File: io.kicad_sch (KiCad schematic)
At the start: 48 parts

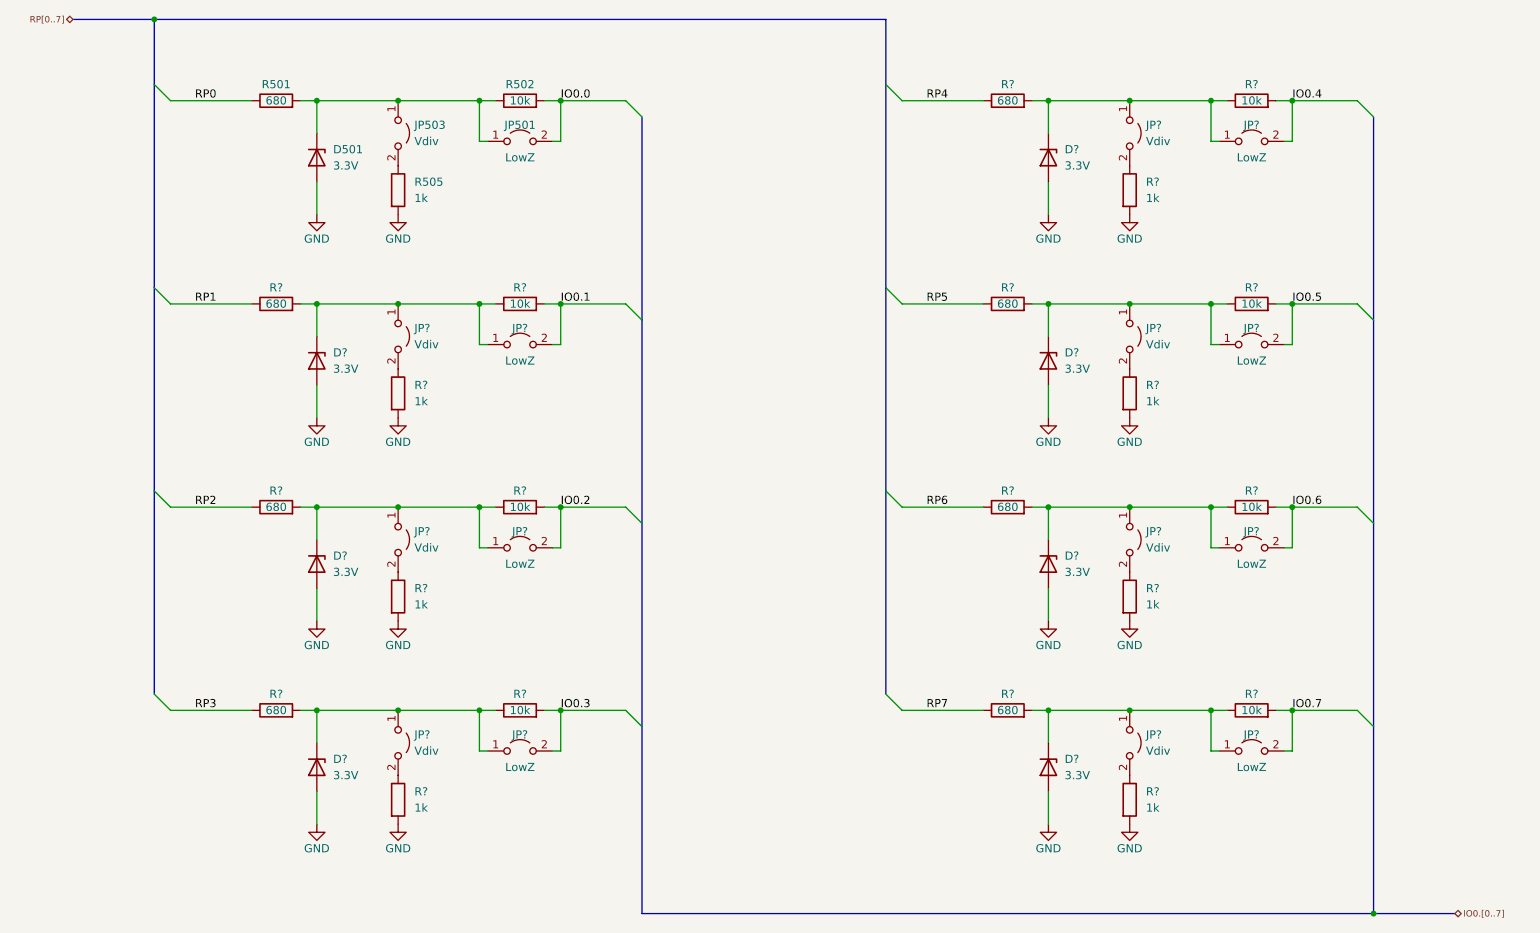
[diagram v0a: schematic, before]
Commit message: started routing
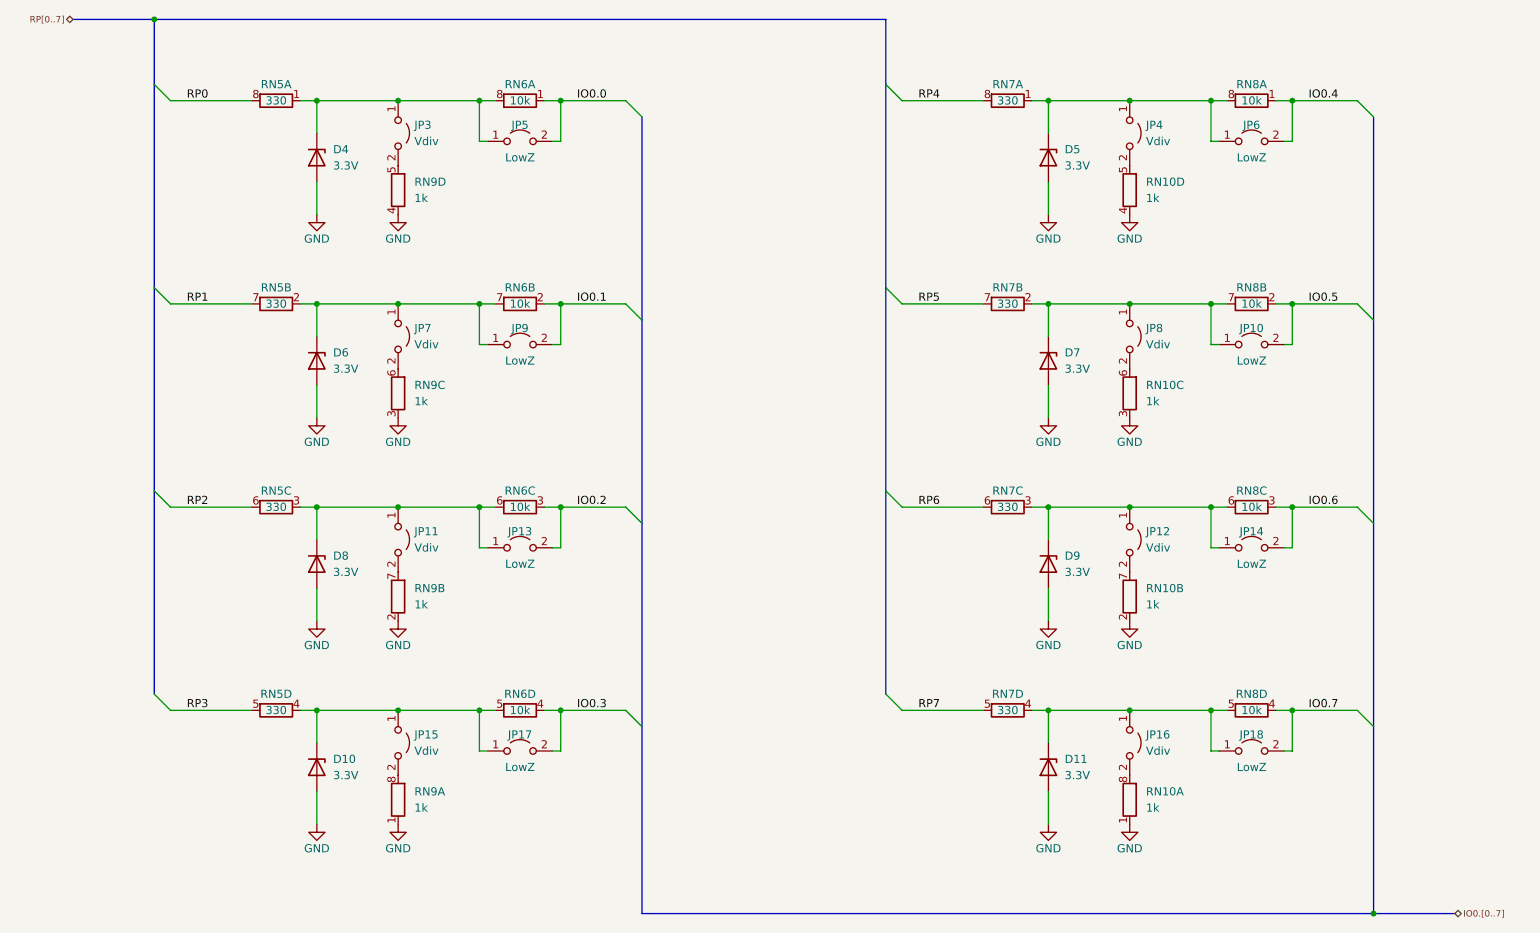
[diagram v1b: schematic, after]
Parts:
- removed D? (x4): 3.3V, symbol Device:D_Zener
- removed JP? (x4): LowZ, symbol Jumper:Jumper_2_Open
- removed JP? (x4): Vdiv, symbol Jumper:Jumper_2_Open
- removed R501, R? (x7): 680, symbol Device:R
- removed R502, R? (x7): 10k, symbol Device:R
- removed R505, R? (x7): 1k, symbol Device:R
- added D11, D5, D7, D9: 3.3V, Diode_SMD:D_SOD-123, symbol Device:D_Zener
- added JP10, JP14, JP18, JP6: LowZ, Jumper:SolderJumper-2_P1.3mm_Open_TrianglePad1.0x1.5mm, symbol Jumper:Jumper_2_Open
- added JP12, JP16, JP4, JP8: Vdiv, Jumper:SolderJumper-2_P1.3mm_Open_TrianglePad1.0x1.5mm, symbol Jumper:Jumper_2_Open
- added RN10, RN9: 1k, Resistor_SMD:R_Array_Convex_4x0603, symbol Device:R_Pack04_Split
- added RN5, RN7: 330, Resistor_SMD:R_Array_Convex_4x0603, symbol Device:R_Pack04_Split
- added RN6, RN8: 10k, Resistor_SMD:R_Array_Convex_4x0603, symbol Device:R_Pack04_Split
- D10, D6, D8: renamed from D?; footprint (none) -> Diode_SMD:D_SOD-123
- D4: renamed from D501; footprint (none) -> Diode_SMD:D_SOD-123
- JP11, JP13, JP15, JP17, JP7, JP9: renamed from JP?; footprint (none) -> Jumper:SolderJumper-2_P1.3mm_Open_TrianglePad1.0x1.5mm
- JP3: renamed from JP503; footprint (none) -> Jumper:SolderJumper-2_P1.3mm_Open_TrianglePad1.0x1.5mm
- JP5: renamed from JP501; footprint (none) -> Jumper:SolderJumper-2_P1.3mm_Open_TrianglePad1.0x1.5mm
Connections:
- net GND: now also D11.2 (A), D5.2 (A), D7.2 (A), D9.2 (A), RN10.1 (R1.1), RN10.2 (R2.1), RN10.3 (R3.1), RN10.4 (R4.1), RN9.1 (R1.1), RN9.2 (R2.1), RN9.3 (R3.1), RN9.4 (R4.1)
- net IO0.0: now also RN6.1 (R1.1)
- net IO0.1: now also RN6.2 (R2.1)
- net IO0.2: now also RN6.3 (R3.1)
- net IO0.3: now also RN6.4 (R4.1)
- net IO0.4: now also JP6.2 (B), RN8.1 (R1.1)
- net IO0.5: now also JP10.2 (B), RN8.2 (R2.1)
- net IO0.6: now also JP14.2 (B), RN8.3 (R3.1)
- net IO0.7: now also JP18.2 (B), RN8.4 (R4.1)
- net RP0: now also RN5.8 (R1.2)
- net RP1: now also RN5.7 (R2.2)
- net RP2: now also RN5.6 (R3.2)
- net RP3: now also RN5.5 (R4.2)
- net RP4: now also RN7.8 (R1.2)
- net RP5: now also RN7.7 (R2.2)
- net RP6: now also RN7.6 (R3.2)
- net RP7: now also RN7.5 (R4.2)
- net at D8.1 (K), JP11.1 (A), JP13.1 (A): now also RN5.3 (R3.1), RN6.6 (R3.2)
- net at JP11.2 (B): now also RN9.7 (R2.2)
- net at D10.1 (K), JP15.1 (A), JP17.1 (A): now also RN5.4 (R4.1), RN6.5 (R4.2)
- net at JP15.2 (B): now also RN9.8 (R1.2)
- net at JP3.2 (B): now also RN9.5 (R4.2)
- net at JP7.2 (B): now also RN9.6 (R3.2)
- net at D6.1 (K), JP7.1 (A), JP9.1 (A): now also RN5.2 (R2.1), RN6.7 (R2.2)
- net at D4.1 (K), JP3.1 (A), JP5.1 (A): now also RN5.1 (R1.1), RN6.8 (R1.2)
- new net: JP12.2 (B), RN10.7 (R2.2)
- new net: JP16.2 (B), RN10.8 (R1.2)
- new net: D5.1 (K), JP4.1 (A), JP6.1 (A), RN7.1 (R1.1), RN8.8 (R1.2)
- new net: JP4.2 (B), RN10.5 (R4.2)
- new net: D11.1 (K), JP16.1 (A), JP18.1 (A), RN7.4 (R4.1), RN8.5 (R4.2)
- new net: D9.1 (K), JP12.1 (A), JP14.1 (A), RN7.3 (R3.1), RN8.6 (R3.2)
- new net: D7.1 (K), JP10.1 (A), JP8.1 (A), RN7.2 (R2.1), RN8.7 (R2.2)
- new net: JP8.2 (B), RN10.6 (R3.2)
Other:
- title: (none) -> [canbrd] CAN/RS485 IO board
